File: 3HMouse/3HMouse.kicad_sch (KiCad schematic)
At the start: 85 parts, among them J1 USB_C_Receptacle_USB2.0, SW1 CherryMX, SW10 CherryMX, SW11 CherryMX, SW12 CherryMX, SW13 CherryMX, SW14 CherryMX, SW15 CherryMX, SW16 CherryMX, SW17 CherryMX, SW18 CherryMX, SW19 CherryMX, SW2 CherryMX, SW20 CherryMX, SW21 CherryMX, SW22 CherryMX, SW23 CherryMX, SW24 CherryMX, SW25 CherryMX, SW26 CherryMX, SW27 CherryMX, SW28 CherryMX, SW29 CherryMX, SW3 CherryMX, SW30 RotaryEncoder, SW31 RotaryEncoder, SW32 Reset, SW4 CherryMX, SW5 CherryMX, SW6 CherryMX, SW7 CherryMX, SW8 CherryMX, SW9 CherryMX, U1 AT90USB1286-A, U2 USBLC6-2SC6, Y1 16 MHz

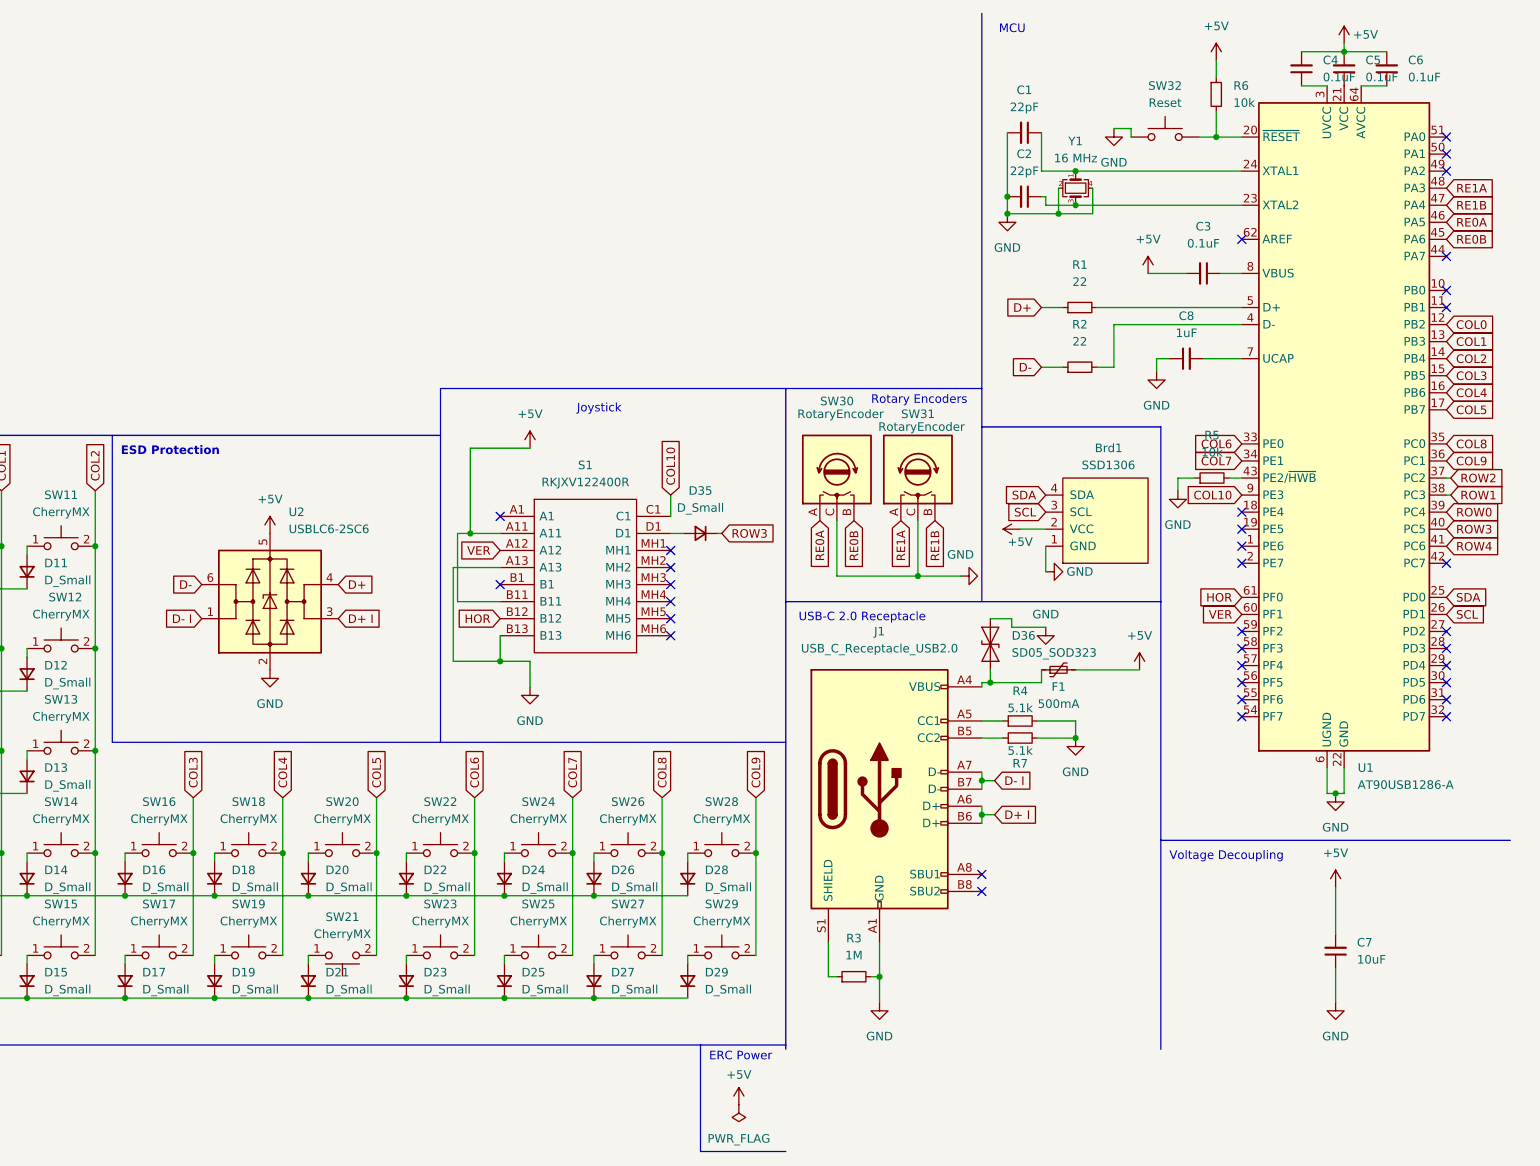
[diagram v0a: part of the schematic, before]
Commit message: v0.4.0 final
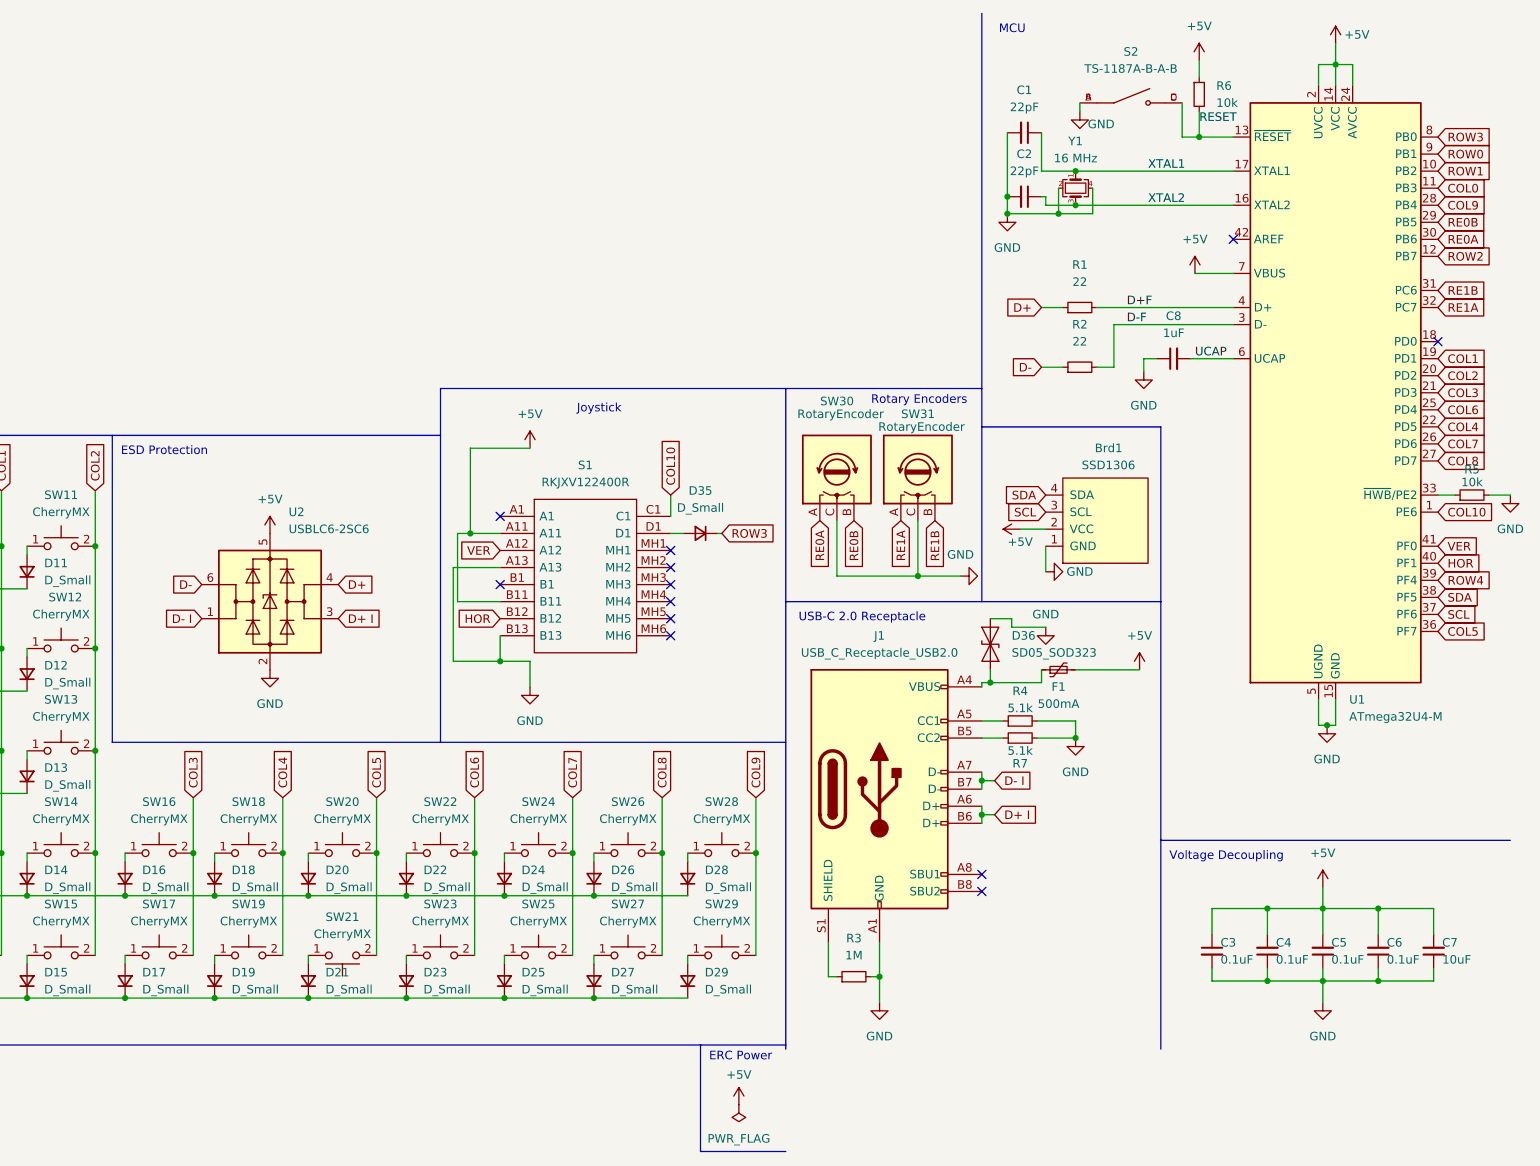
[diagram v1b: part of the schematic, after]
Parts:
- removed SW32: Reset, random-keyboard-parts:SKQG-1155865, symbol Switch:SW_Push
- removed U1: AT90USB1286-A, Package_QFP:TQFP-64_14x14mm_P0.8mm, symbol MCU_Microchip_AVR:AT90USB1286-A
- added S2: TS-1187A-B-A-B, SW_TS-1187A-B-A-B:SW_TS-1187A-B-A-B, symbol TS-1187A-B-A-B:TS-1187A-B-A-B
- added U1: ATmega32U4-M, Package_DFN_QFN:QFN-44-1EP_7x7mm_P0.5mm_EP5.2x5.2mm, symbol MCU_Microchip_ATmega:ATmega32U4-M
- J1: footprint Connector_USB:USB_C_Receptacle_GCT_USB4085 -> USB_C_Receptacle_GT-USB-7010:USB_C_Receptacle_GT-USB-7010
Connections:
- net +5V: now also C3.1, U1.14 (VCC), U1.2 (UVCC), U1.24 (AVCC), U1.34 (VCC), U1.44 (AVCC), U1.7 (VBUS); no longer C3.2
- net COL0: now also U1.11 (PB3)
- net COL1: now also U1.19 (PD1)
- net COL10: now also U1.1 (PE6)
- net COL2: now also U1.20 (PD2)
- net COL3: now also U1.21 (PD3)
- net COL4: now also U1.22 (PD5)
- net COL5: now also U1.36 (PF7)
- net COL6: now also U1.25 (PD4)
- net COL7: now also U1.26 (PD6)
- net COL8: now also U1.27 (PD7)
- net COL9: now also U1.28 (PB4)
- net GND: now also C3.2, C4.1, C5.1, C6.1, R5.2, S2.A, S2.B, U1.15 (GND), U1.23 (GND), U1.35 (GND), U1.43 (GND), U1.45 (GND), U1.5 (UGND); no longer R5.1
- net HOR: now also U1.40 (PF1)
- net RE0A: now also U1.30 (PB6)
- net RE0B: now also U1.29 (PB5)
- net RE1A: now also U1.32 (PC7)
- net RE1B: now also U1.31 (PC6)
- net ROW0: now also U1.9 (PB1)
- net ROW1: now also U1.10 (PB2)
- net ROW2: now also U1.12 (PB7)
- net ROW3: now also U1.8 (PB0)
- net ROW4: now also U1.39 (PF4)
- net SCL: now also U1.37 (PF6)
- net SDA: now also U1.38 (PF5)
- net VER: now also U1.41 (PF0)
- net XTAL1: now reaches C1.1, Y1.1
- net XTAL1: now also U1.17 (XTAL1)
- net D-F: now reaches R2.2
- net D-F: now also U1.3 (D-)
- net XTAL2: now reaches C2.1, Y1.3
- net XTAL2: now also U1.16 (XTAL2)
- net RESET: now reaches R6.2
- net RESET: now also S2.C, S2.D, U1.13 (~{RESET})
- net D+F: now reaches R1.2
- net D+F: now also U1.4 (D+)
- net UCAP: now reaches C8.2
- net UCAP: now also U1.6 (UCAP)
- new net: R5.1, U1.33 (~{HWB}/PE2)
- no-connect marks 34 -> 12
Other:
- moved on the sheet: C3, C4, C5, C6, C7, C8, R5, R6

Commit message: Placements done for v2
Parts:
- removed D20, D21, D22, D23, D24, D25, D26, D27, D28, D29, D35: D_Small, Diode_SMD:D_SOD-123, symbol Device:D_Small
- removed SW20, SW21, SW22, SW23, SW24, SW25, SW26, SW27, SW28, SW29: CherryMX, MX_Only:MXOnly-1U-NoLED, symbol CherryMX:CherryMX
- removed SW30, SW31: RotaryEncoder, Keebio-Parts:RotaryEncoder_EC11, symbol Device:RotaryEncoder
- added D0_3, D1_3, D2_3, D5_0, D5_1, D5_2, D5_3, D5_4, D6_0, D6_1, D6_2, D6_3, D6_4: D_Small, Diode_SMD:D_SOD-123, symbol Device:D_Small
- added DL0_0, DL0_1, DL0_2, DL1_0, DL1_1, DL1_2, DL2_0, DL2_1, DL2_2, DL3_0, DL3_1, DL3_2, DL3_3, DL3_4, DL4_0, DL4_1, DL4_2, DL4_3, DL4_4, DL5_0, DL5_1, DL5_2, DL5_3, DL5_4, DL6_0, DL6_1, DL6_2, DL6_3, DL6_4: SK6805-EC15, HLibrary:SK6805-EC15, symbol HLibrary:SK6805-EC15
- added R8: 500, Resistor_SMD:R_0805_2012Metric, symbol Device:R_Small
- added RE1, RE2: RotaryEncoder_Switch, Rotary_Encoder:RotaryEncoder_Alps_EC11E-Switch_Vertical_H20mm, symbol Device:RotaryEncoder_Switch
- added SW5_0, SW5_1, SW5_2, SW5_3, SW5_4, SW6_0, SW6_1, SW6_2, SW6_3, SW6_4: CherryMX, MX_Only:MXOnly-1U-Hotswap, symbol CherryMX:CherryMX
- SW0_0: renamed from SW1; footprint MX_Only:MXOnly-1U-NoLED -> MX_Only:MXOnly-1U-Hotswap
- SW0_1: renamed from SW6; footprint MX_Only:MXOnly-1U-NoLED -> MX_Only:MXOnly-1U-Hotswap
- SW0_2: renamed from SW11; footprint MX_Only:MXOnly-1U-NoLED -> MX_Only:MXOnly-1U-Hotswap
- SW1_0: renamed from SW2; footprint MX_Only:MXOnly-1U-NoLED -> MX_Only:MXOnly-1U-Hotswap
- SW1_1: renamed from SW7; footprint MX_Only:MXOnly-1U-NoLED -> MX_Only:MXOnly-1U-Hotswap
- SW1_2: renamed from SW12; footprint MX_Only:MXOnly-1U-NoLED -> MX_Only:MXOnly-1U-Hotswap
- SW2_0: renamed from SW3; footprint MX_Only:MXOnly-1U-NoLED -> MX_Only:MXOnly-1U-Hotswap
- SW2_1: renamed from SW8; footprint MX_Only:MXOnly-1U-NoLED -> MX_Only:MXOnly-1U-Hotswap
- SW2_2: renamed from SW13; footprint MX_Only:MXOnly-1U-NoLED -> MX_Only:MXOnly-1U-Hotswap
- SW3_0: renamed from SW4; footprint MX_Only:MXOnly-1.5U-NoLED -> MX_Only:MXOnly-1U-Hotswap
- SW3_1: renamed from SW9; footprint MX_Only:MXOnly-1U-NoLED -> MX_Only:MXOnly-1U-Hotswap
- SW3_2: renamed from SW14; footprint MX_Only:MXOnly-1U-NoLED -> MX_Only:MXOnly-1U-Hotswap
- SW3_3: renamed from SW16; footprint MX_Only:MXOnly-1U-NoLED -> MX_Only:MXOnly-1U-Hotswap
- SW3_4: renamed from SW18; footprint MX_Only:MXOnly-1U-NoLED -> MX_Only:MXOnly-1U-Hotswap
- SW4_0: renamed from SW5; footprint MX_Only:MXOnly-1.25U-NoLED -> MX_Only:MXOnly-1U-Hotswap
- SW4_1: renamed from SW10; footprint MX_Only:MXOnly-1.25U-NoLED -> MX_Only:MXOnly-1U-Hotswap
- SW4_2: renamed from SW15; footprint MX_Only:MXOnly-1U-NoLED -> MX_Only:MXOnly-1U-Hotswap
- SW4_3: renamed from SW17; footprint MX_Only:MXOnly-1U-NoLED -> MX_Only:MXOnly-1U-Hotswap
- SW4_4: renamed from SW19; footprint MX_Only:MXOnly-1U-NoLED -> MX_Only:MXOnly-1U-Hotswap
- renumbered D1 to D0_0, D6 to D0_1, D11 to D0_2, D2 to D1_0, D7 to D1_1, D12 to D1_2, D3 to D2_0, D8 to D2_1, D13 to D2_2, D4 to D3_0, D9 to D3_1, D14 to D3_2, D16 to D3_3, D18 to D3_4, D5 to D4_0, D10 to D4_1, D15 to D4_2, D17 to D4_3, D19 to D4_4
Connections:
- net +5V: now also DL0_0.2 (VDD), DL0_1.2 (VDD), DL0_2.2 (VDD), DL1_0.2 (VDD), DL1_1.2 (VDD), DL1_2.2 (VDD), DL2_0.2 (VDD), DL2_1.2 (VDD), DL2_2.2 (VDD), DL3_0.2 (VDD), DL3_1.2 (VDD), DL3_2.2 (VDD), DL3_3.2 (VDD), DL3_4.2 (VDD), DL4_0.2 (VDD), DL4_1.2 (VDD), DL4_2.2 (VDD), DL4_3.2 (VDD), DL4_4.2 (VDD), DL5_0.2 (VDD), DL5_1.2 (VDD), DL5_2.2 (VDD), DL5_3.2 (VDD), DL5_4.2 (VDD), DL6_0.2 (VDD), DL6_1.2 (VDD), DL6_2.2 (VDD), DL6_3.2 (VDD), DL6_4.2 (VDD)
- net COL0: now also SW5_0.2, SW6_0.2
- net COL1: now also SW5_1.2, SW6_1.2
- net COL2: now also SW5_2.2, SW6_2.2
- net COL3: now also S1.C1, RE1.S1, RE2.S1, SW5_3.2, SW6_3.2
- net COL4: now also SW5_4.2, SW6_4.2
- net GND: now also DL0_0.4 (GND), DL0_1.4 (GND), DL0_2.4 (GND), DL1_0.4 (GND), DL1_1.4 (GND), DL1_2.4 (GND), DL2_0.4 (GND), DL2_1.4 (GND), DL2_2.4 (GND), DL3_0.4 (GND), DL3_1.4 (GND), DL3_2.4 (GND), DL3_3.4 (GND), DL3_4.4 (GND), DL4_0.4 (GND), DL4_1.4 (GND), DL4_2.4 (GND), DL4_3.4 (GND), DL4_4.4 (GND), DL5_0.4 (GND), DL5_1.4 (GND), DL5_2.4 (GND), DL5_3.4 (GND), DL5_4.4 (GND), DL6_0.4 (GND), DL6_1.4 (GND), DL6_2.4 (GND), DL6_3.4 (GND), DL6_4.4 (GND), RE1.C, RE2.C
- net RE0A: now also RE1.A
- net RE0B: now also RE1.B
- net RE1A: now also RE2.A
- net RE1B: now also RE2.B
- net ROW0: now also D0_3.1 (K)
- net ROW1: now also D1_3.1 (K)
- net ROW2: now also D2_3.1 (K)
- net LED: now reaches U1.18 (PD0)
- net LED: now also R8.1
- net at S1.D1: now also D0_3.2 (A)
- net COL10: no longer names the net of U1.1 (PE6)
- net COL10: no longer S1.C1
- net COL5: no longer names the net of U1.36 (PF7)
- net COL6 renamed ROW6
- net ROW6: now also D6_0.1 (K), D6_1.1 (K), D6_2.1 (K), D6_3.1 (K), D6_4.1 (K)
- net COL7: no longer names the net of U1.26 (PD6)
- net COL8: no longer names the net of U1.27 (PD7)
- net COL9 renamed ROW5
- net ROW5: now also D5_0.1 (K), D5_1.1 (K), D5_2.1 (K), D5_3.1 (K), D5_4.1 (K)
- new net: D6_2.2 (A), SW6_2.1
- new net: DL2_1.3 (DOUT), DL2_2.1 (DIN)
- new net: DL2_2.3 (DOUT), DL3_0.1 (DIN)
- new net: D6_3.2 (A), SW6_3.1
- new net: DL3_3.3 (DOUT), DL3_4.1 (DIN)
- new net: DL3_4.3 (DOUT), DL4_0.1 (DIN)
- new net: DL1_0.3 (DOUT), DL1_1.1 (DIN)
- new net: DL1_1.3 (DOUT), DL1_2.1 (DIN)
- new net: D5_0.2 (A), SW5_0.1
- new net: D6_4.2 (A), SW6_4.1
- new net: DL4_4.3 (DOUT), DL5_0.1 (DIN)
- new net: DL5_0.3 (DOUT), DL5_1.1 (DIN)
- new net: DL0_2.3 (DOUT), DL1_0.1 (DIN)
- new net: D6_1.2 (A), SW6_1.1
- new net: D2_3.2 (A), RE2.S2
- new net: DL4_0.3 (DOUT), DL4_1.1 (DIN)
- new net: DL4_1.3 (DOUT), DL4_2.1 (DIN)
- new net: DL0_0.1 (DIN), R8.2
- new net: DL0_0.3 (DOUT), DL0_1.1 (DIN)
- new net: DL5_2.3 (DOUT), DL5_3.1 (DIN)
- new net: DL5_3.3 (DOUT), DL5_4.1 (DIN)
- new net: DL3_0.3 (DOUT), DL3_1.1 (DIN)
- new net: DL4_2.3 (DOUT), DL4_3.1 (DIN)
- new net: DL4_3.3 (DOUT), DL4_4.1 (DIN)
- new net: D1_3.2 (A), RE1.S2
- new net: DL1_2.3 (DOUT), DL2_0.1 (DIN)
- new net: DL2_0.3 (DOUT), DL2_1.1 (DIN)
- new net: D6_0.2 (A), SW6_0.1
- new net: DL6_2.3 (DOUT), DL6_3.1 (DIN)
- new net: DL6_3.3 (DOUT), DL6_4.1 (DIN)
- new net: DL3_1.3 (DOUT), DL3_2.1 (DIN)
- new net: D5_2.2 (A), SW5_2.1
- new net: D5_3.2 (A), SW5_3.1
- new net: D5_1.2 (A), SW5_1.1
- new net: DL0_1.3 (DOUT), DL0_2.1 (DIN)
- new net: D5_4.2 (A), SW5_4.1
- new net: DL5_4.3 (DOUT), DL6_0.1 (DIN)
- new net: DL3_2.3 (DOUT), DL3_3.1 (DIN)
- new net: DL6_0.3 (DOUT), DL6_1.1 (DIN)
- new net: DL6_1.3 (DOUT), DL6_2.1 (DIN)
- new net: DL5_1.3 (DOUT), DL5_2.1 (DIN)
- no-connect marks 12 -> 16
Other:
- note added: "RGB LEDs"
- note removed: "3HMouse"
- moved on the sheet: Brd1, C1, C2, C3, C4, C5, C6, C7, C8, D0_0, D0_1, D0_2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
